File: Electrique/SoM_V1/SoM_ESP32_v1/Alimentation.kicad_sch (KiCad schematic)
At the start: 1 part

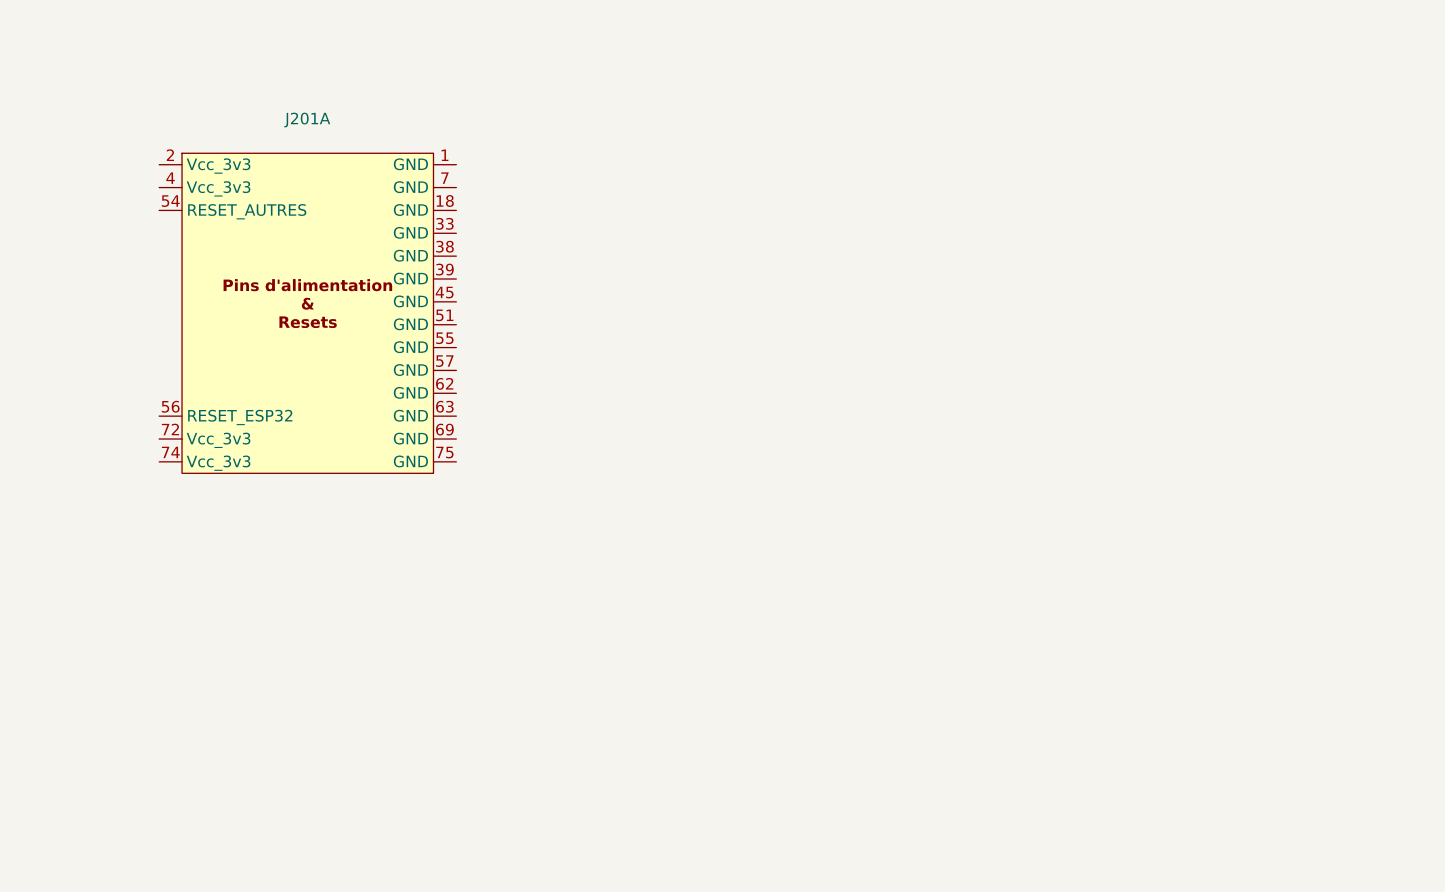
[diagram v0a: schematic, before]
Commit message: push pcb
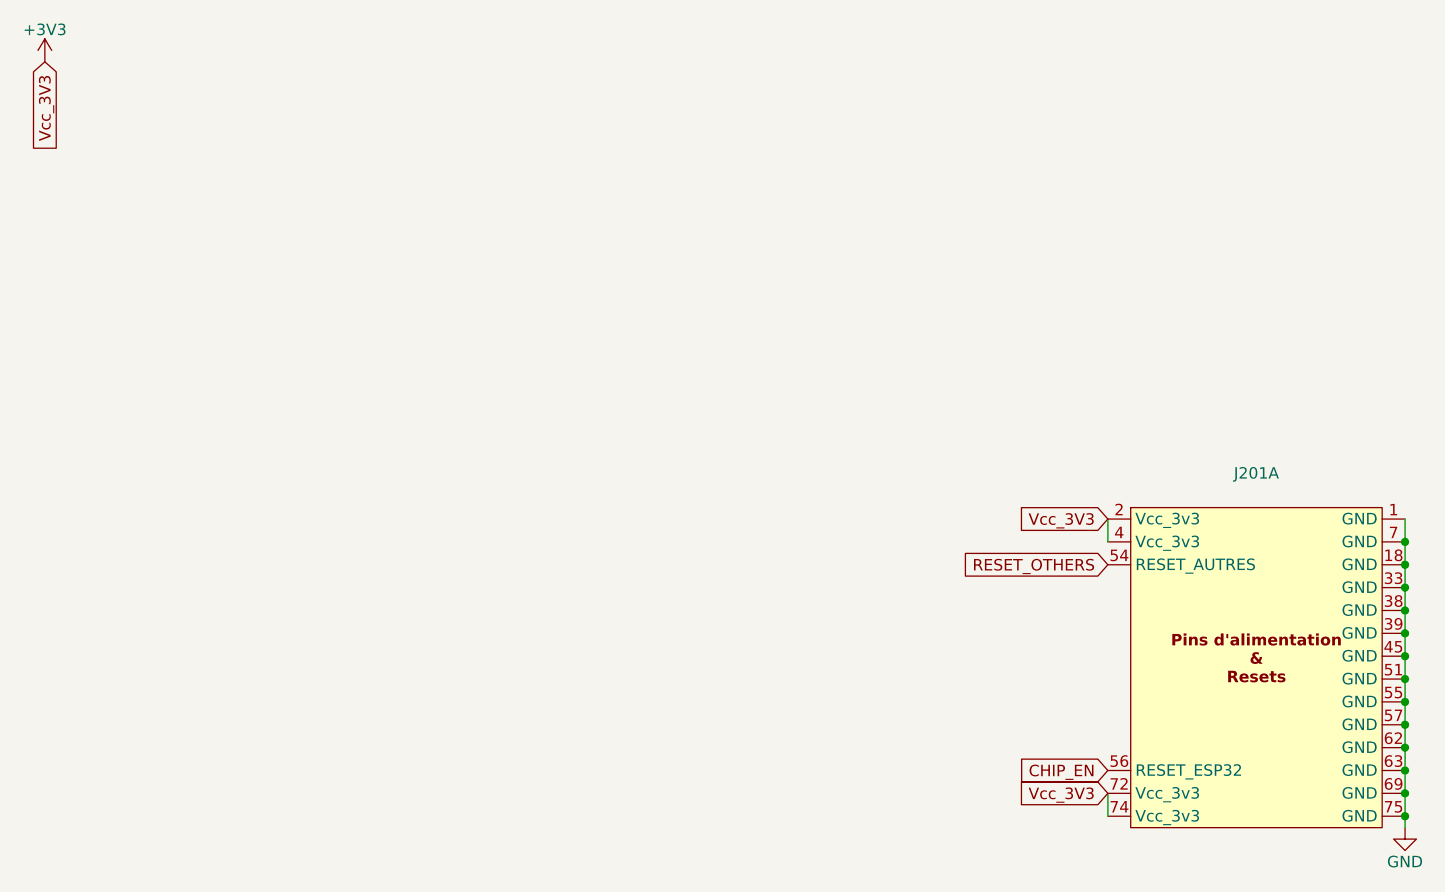
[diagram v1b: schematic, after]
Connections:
- net GND: now reaches J201.1 (GND)
- net GND: now also J201.18 (GND), J201.33 (GND), J201.38 (GND), J201.39 (GND), J201.45 (GND), J201.51 (GND), J201.55 (GND), J201.57 (GND), J201.62 (GND), J201.63 (GND), J201.69 (GND), J201.7 (GND), J201.75 (GND)
- net +3V3: now reaches J201.2 (Vcc_3v3)
- net +3V3: now also J201.4 (Vcc_3v3), J201.72 (Vcc_3v3), J201.74 (Vcc_3v3)
- net RESET_OTHERS: now reaches J201.54 (RESET_AUTRES)
- net CHIP_EN: now reaches J201.56 (RESET_ESP32)
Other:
- moved on the sheet: J201A
